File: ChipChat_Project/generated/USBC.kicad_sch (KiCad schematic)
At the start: 4 parts

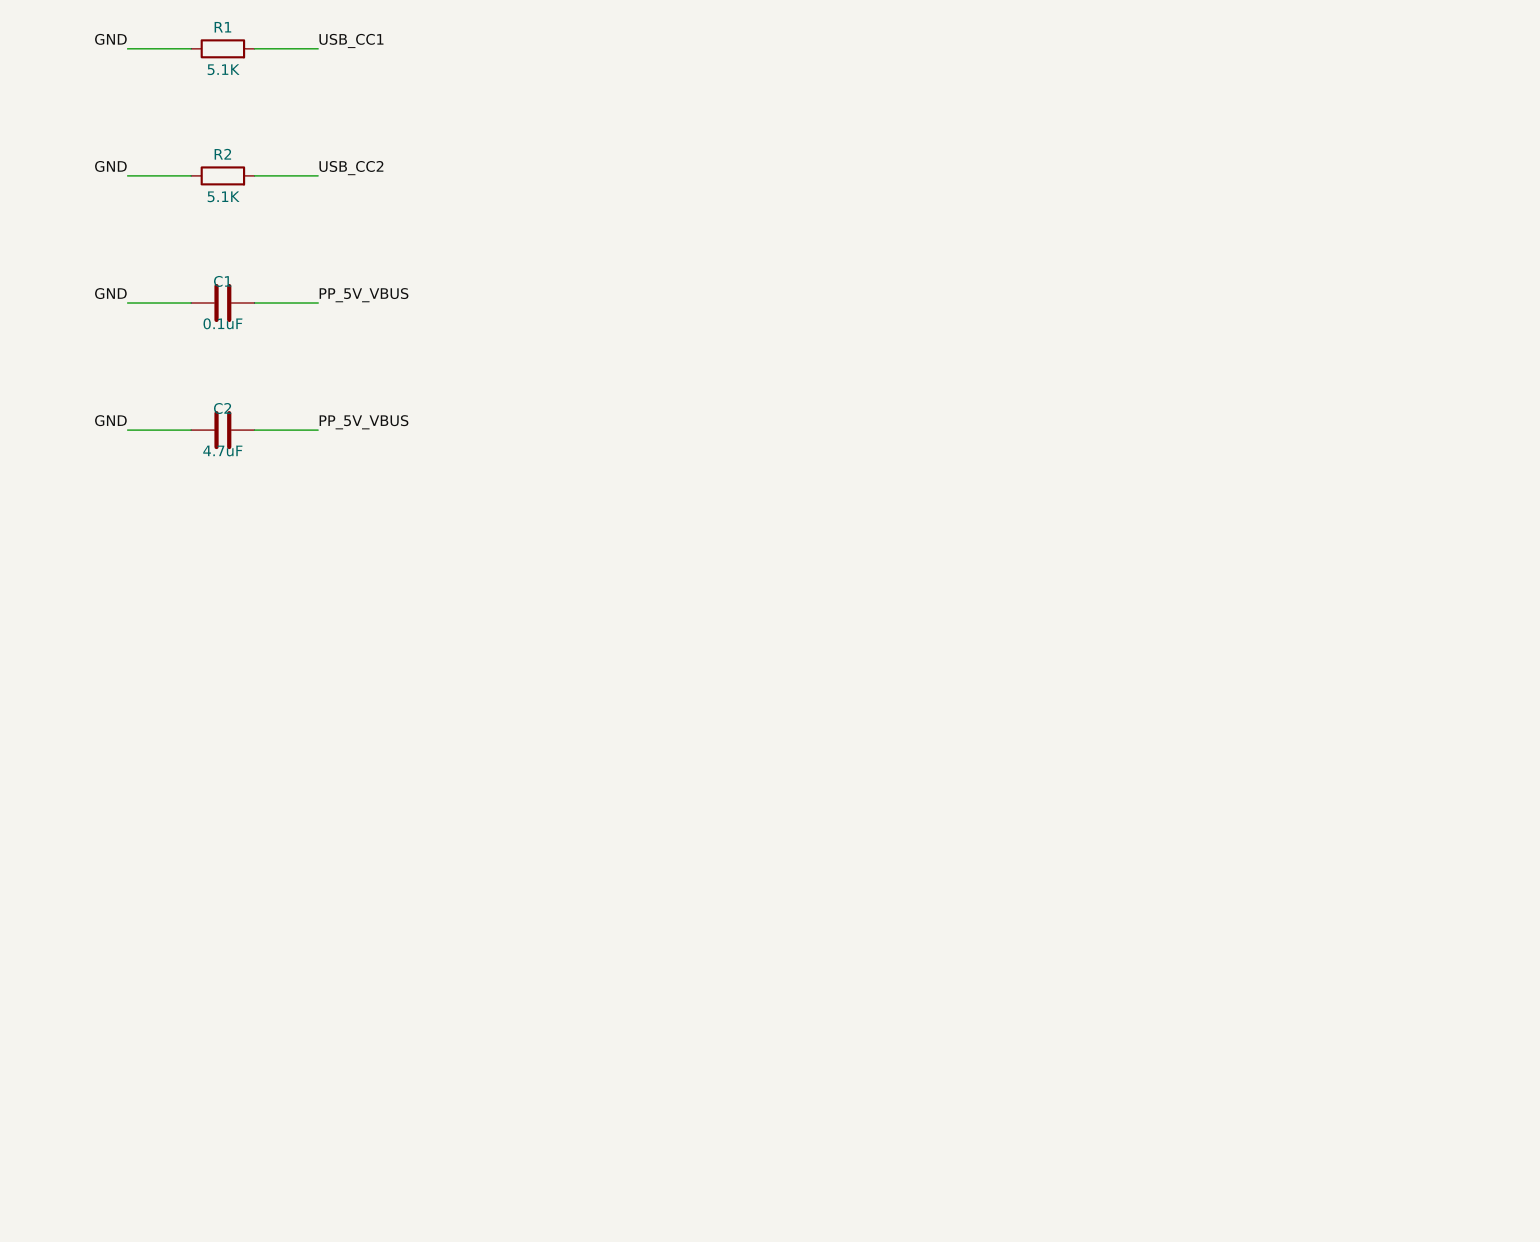
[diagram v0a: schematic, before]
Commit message: 💾 snapshot 2026-02-23_00-19-22
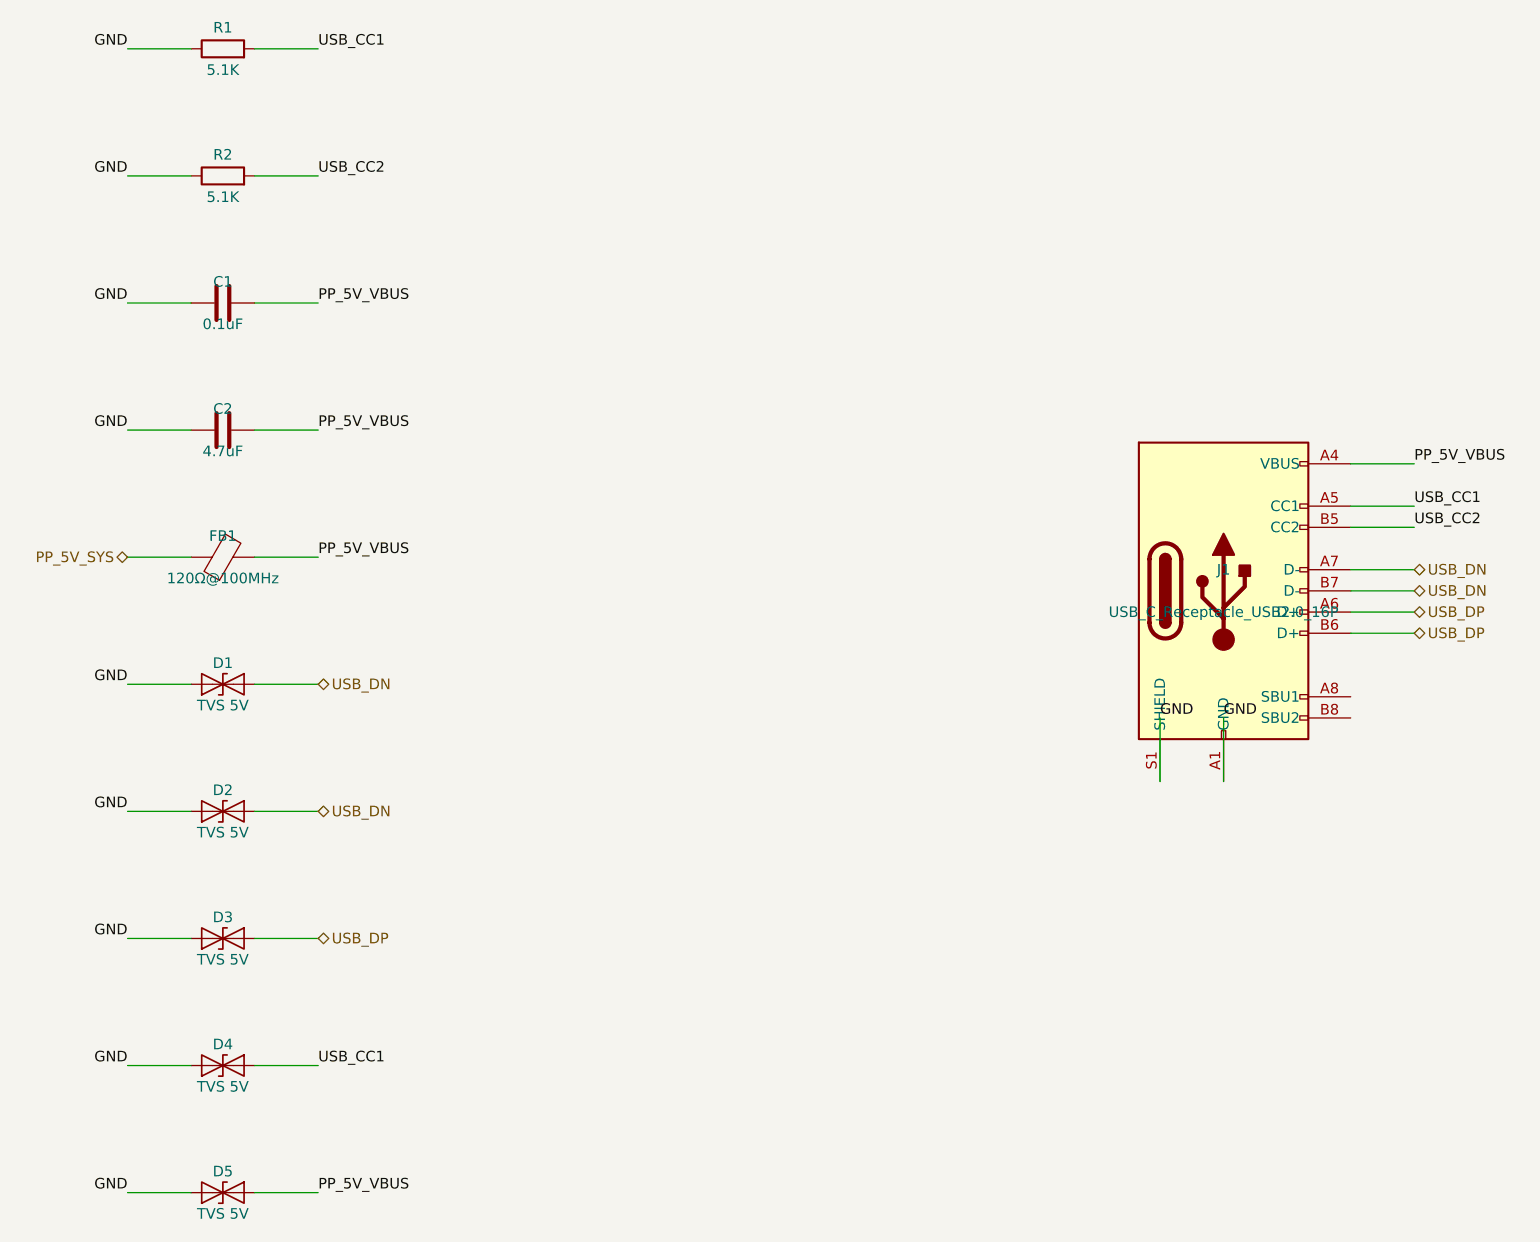
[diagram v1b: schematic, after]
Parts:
- added D1, D2, D3, D4, D5: TVS 5V, symbol SD05_SOD323
- added FB1: 120Ω@100MHz, symbol FerriteBead
- added J1: USB_C_Receptacle_USB2.0_16P, symbol USB_C_Receptacle_USB2.0_16P
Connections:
- net GND: now also D1.2 (A2), D2.2 (A2), D3.2 (A2), D4.2 (A2), D5.2 (A2), J1.A1 (GND), J1.A12 (GND), J1.B1 (GND), J1.B12 (GND), J1.S1 (SHIELD)
- net PP_5V_VBUS: now also D5.1 (A1), FB1.2, J1.A4 (VBUS), J1.A9 (VBUS), J1.B4 (VBUS), J1.B9 (VBUS)
- net USB_CC1: now also D4.1 (A1), J1.A5 (CC1)
- net USB_CC2: now also J1.B5 (CC2)
- new net PP_5V_SYS: FB1.1
- new net USB_DN: D1.1 (A1), D2.1 (A1), J1.A7 (D-), J1.B7 (D-)
- new net USB_DP: D3.1 (A1), J1.A6 (D+), J1.B6 (D+)
